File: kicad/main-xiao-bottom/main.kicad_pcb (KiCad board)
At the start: 2 copper layers, 41 x 41.5 mm, 23 parts, among them J1 Conn_01x14, J10 Conn_01x01_Pin, J11 Conn_01x01_Pin, J12 Conn_01x01_Pin, J13 Conn_01x01_Pin, J14 Conn_01x05_Socket, J2 Conn_01x14_Socket, J3 Conn_01x01_Pin, J4 Conn_01x03_Socket, J5 Conn_01x06, J6 Conn_01x08, J7 Conn_01x01_Pin, J8 Conn_01x01_Pin, J9 Conn_01x01_Pin

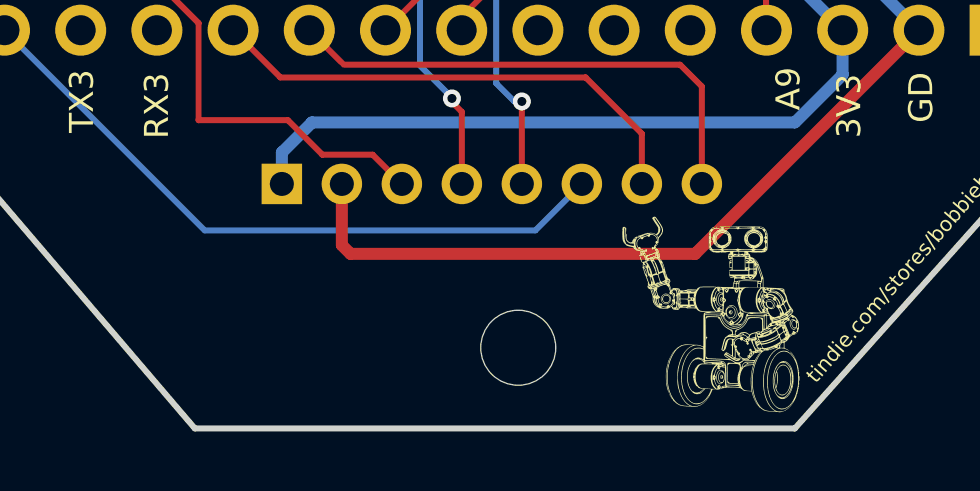
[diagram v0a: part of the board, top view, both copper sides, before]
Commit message: modified:   kicad/main-xiao-bottom/main.kicad_pcb
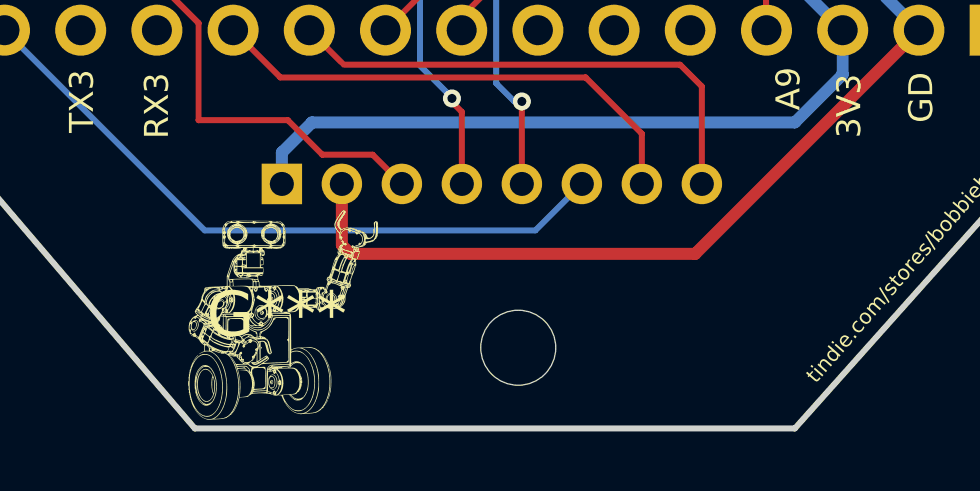
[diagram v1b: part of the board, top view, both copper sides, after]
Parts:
- moved G*** 14.7 mm to (138.0, 102.2)

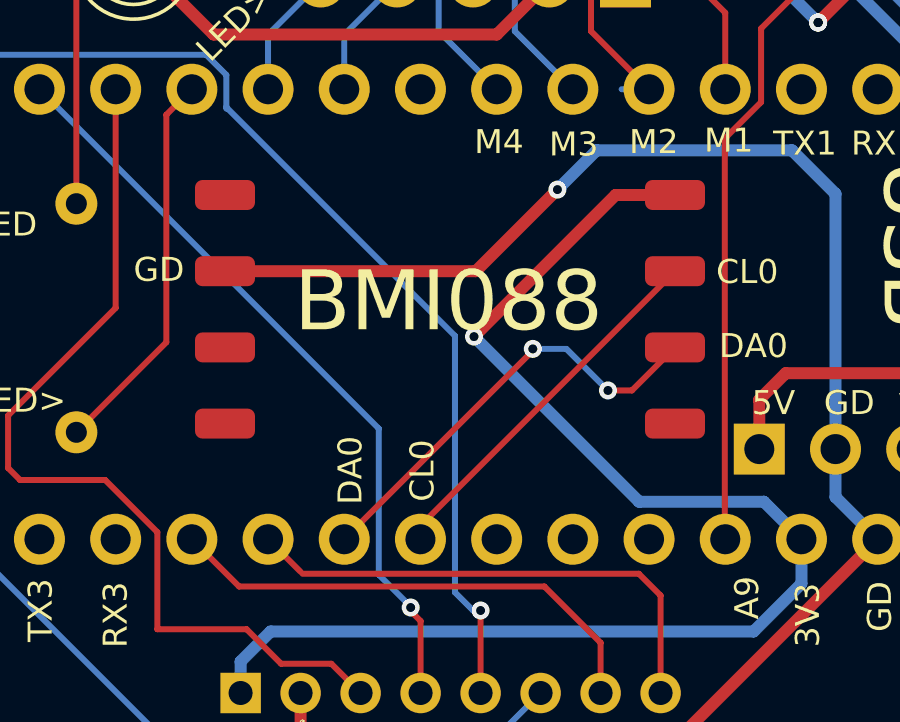
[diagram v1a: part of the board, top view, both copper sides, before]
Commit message: modified:   kicad/main-xiao-bottom/main.kicad_pcb
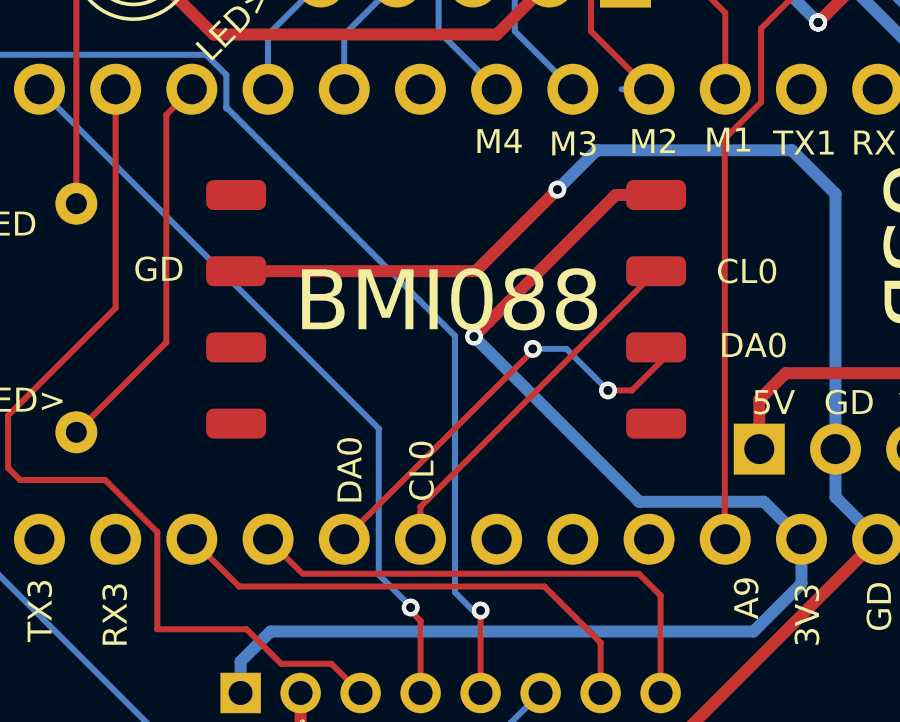
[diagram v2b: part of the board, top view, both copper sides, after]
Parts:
- moved J10 0.63 mm to (152.0, 81.2)
- moved J12 0.63 mm to (152.0, 86.3)
- moved J13 0.63 mm to (152.0, 88.9)
- moved J3 0.37 mm to (138.0, 83.8)
- moved J7 0.37 mm to (138.0, 81.2)
- moved J8 0.37 mm to (138.0, 86.3)
- moved J9 0.37 mm to (138.0, 88.9)
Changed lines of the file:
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@@
 	(footprint "Connector_Wire:SolderWirePad_1x01_SMD_1x2mm"
 		(layer "F.Cu")
-		(at 152.63 81.25 -90)
+		(at 152 81.25 -90)
 		(descr "Wire Pad, Square, SMD Pad,  1mm x 2mm")
 		(tags "MeasurementPoint Square SMDPad 1mmx2mm ")
@@
 	(footprint "Connector_Wire:SolderWirePad_1x01_SMD_1x2mm"
 		(layer "F.Cu")
-		(at 152.63 88.87 -90)
+		(at 152 88.87 -90)
 		(descr "Wire Pad, Square, SMD Pad,  1mm x 2mm")
 		(tags "MeasurementPoint Square SMDPad 1mmx2mm ")
@@
 	(footprint "Connector_Wire:SolderWirePad_1x01_SMD_1x2mm"
 		(layer "F.Cu")
-		(at 137.63 83.79 90)
+		(at 138 83.79 90)
 		(descr "Wire Pad, Square, SMD Pad,  1mm x 2mm")
 		(tags "MeasurementPoint Square SMDPad 1mmx2mm ")
@@
 	(footprint "Connector_Wire:SolderWirePad_1x01_SMD_1x2mm"
 		(layer "F.Cu")
-		(at 137.63 81.25 -90)
+		(at 138 81.25 -90)
 		(descr "Wire Pad, Square, SMD Pad,  1mm x 2mm")
 		(tags "MeasurementPoint Square SMDPad 1mmx2mm ")
@@
 		)
 		(pad "1" smd roundrect
-			(at 0 0 270)
+			(at 0 0.63 270)
 			(size 1 2)
 			(layers "F.Cu" "F.Mask")
@@
 	(footprint "Connector_Wire:SolderWirePad_1x01_SMD_1x2mm"
 		(layer "F.Cu")
-		(at 137.63 88.87 -90)
+		(at 138 88.87 -90)
 		(descr "Wire Pad, Square, SMD Pad,  1mm x 2mm")
 		(tags "MeasurementPoint Square SMDPad 1mmx2mm ")
@@
 	(footprint "Connector_Wire:SolderWirePad_1x01_SMD_1x2mm"
 		(layer "F.Cu")
-		(at 137.63 86.33 -90)
+		(at 138 86.33 -90)
 		(descr "Wire Pad, Square, SMD Pad,  1mm x 2mm")
 		(tags "MeasurementPoint Square SMDPad 1mmx2mm ")
@@
 	(footprint "Connector_Wire:SolderWirePad_1x01_SMD_1x2mm"
 		(layer "F.Cu")
-		(at 152.63 86.33 -90)
+		(at 152 86.33 -90)
 		(descr "Wire Pad, Square, SMD Pad,  1mm x 2mm")
 		(tags "MeasurementPoint Square SMDPad 1mmx2mm ")
@@
 	)
 	(segment
-		(start 144.145 92.275)
-		(end 144.145 92.725)
+		(start 144.145 91.645)
+		(end 152 83.79)
 		(width 0.2)
 		(layer "F.Cu")
@@
 	)
 	(segment
-		(start 152.63 83.79)
-		(end 144.145 92.275)
+		(start 144.145 92.725)
+		(end 144.145 91.645)
 		(width 0.2)
 		(layer "F.Cu")

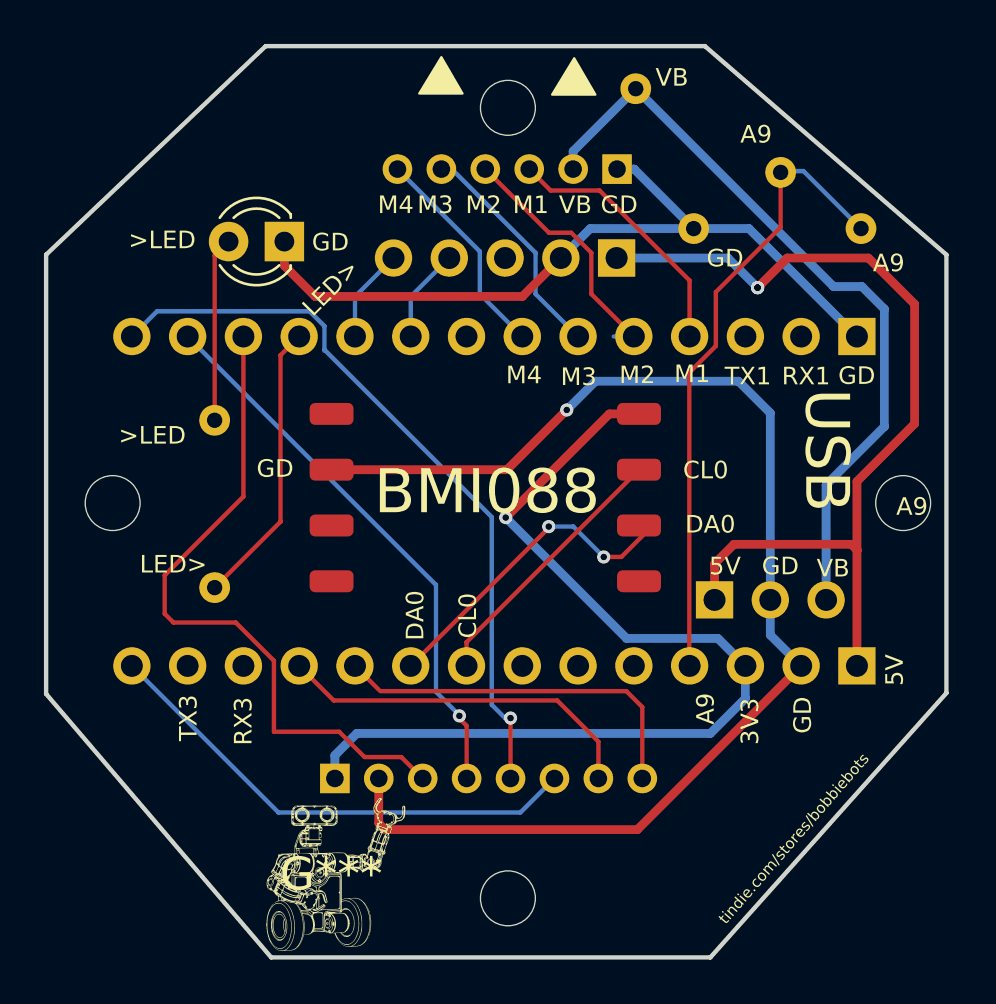
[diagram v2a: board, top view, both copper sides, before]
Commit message: modified:   kicad/main-xiao-bottom/main.kicad_pcb
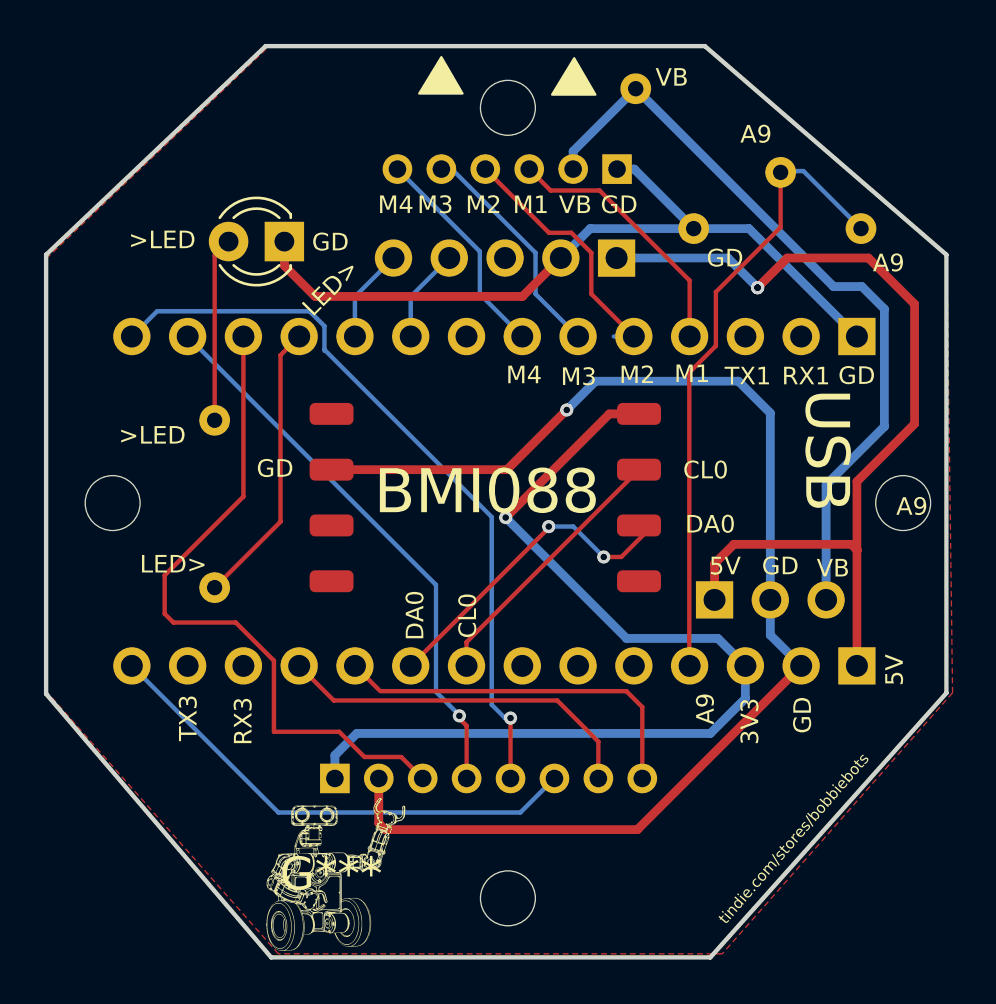
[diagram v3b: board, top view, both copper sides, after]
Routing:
- added copper zone on F.Cu, net /GND
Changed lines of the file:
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@@
 		(net "/SDA0")
+	)
+	(zone
+		(net "/GND")
+		(layer "F.Cu")
+		(hatch edge 0.5)
+		(connect_pads
+			(clearance 0.5)
+		)
+		(min_thickness 0.25)
+		(fill yes
+			(thermal_gap 0.5)
+			(thermal_bridge_width 0.5)
+			(island_removal_mode 0)
+		)
+		(polygon
+			(pts
+				(xy 135.06 64.55) (xy 155.01 64.55) (xy 166.02 74.01) (xy 166.28 93.95) (xy 155.79 105.84) (xy 135.58 105.84)
+				(xy 125 93.87) (xy 125 74.18) (xy 135.13 64.53)
+			)
+		)
 	)
 	(embedded_fonts no)
